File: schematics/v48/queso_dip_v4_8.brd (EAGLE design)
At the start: 41 x 50 mm, 50 parts, among them Q1 FOXSDLF/120-20, U1 PRTR5V0U2X,215, U2 PRTR5V0U2X,215, U3 PRTR5V0U2X,215, U4 PRTR5V0U2X,215, U5 PRTR5V0U2X,215, X1 USB-A-S, X2 USB-A-S, X3 USB-A-S, X4 USB-A-S

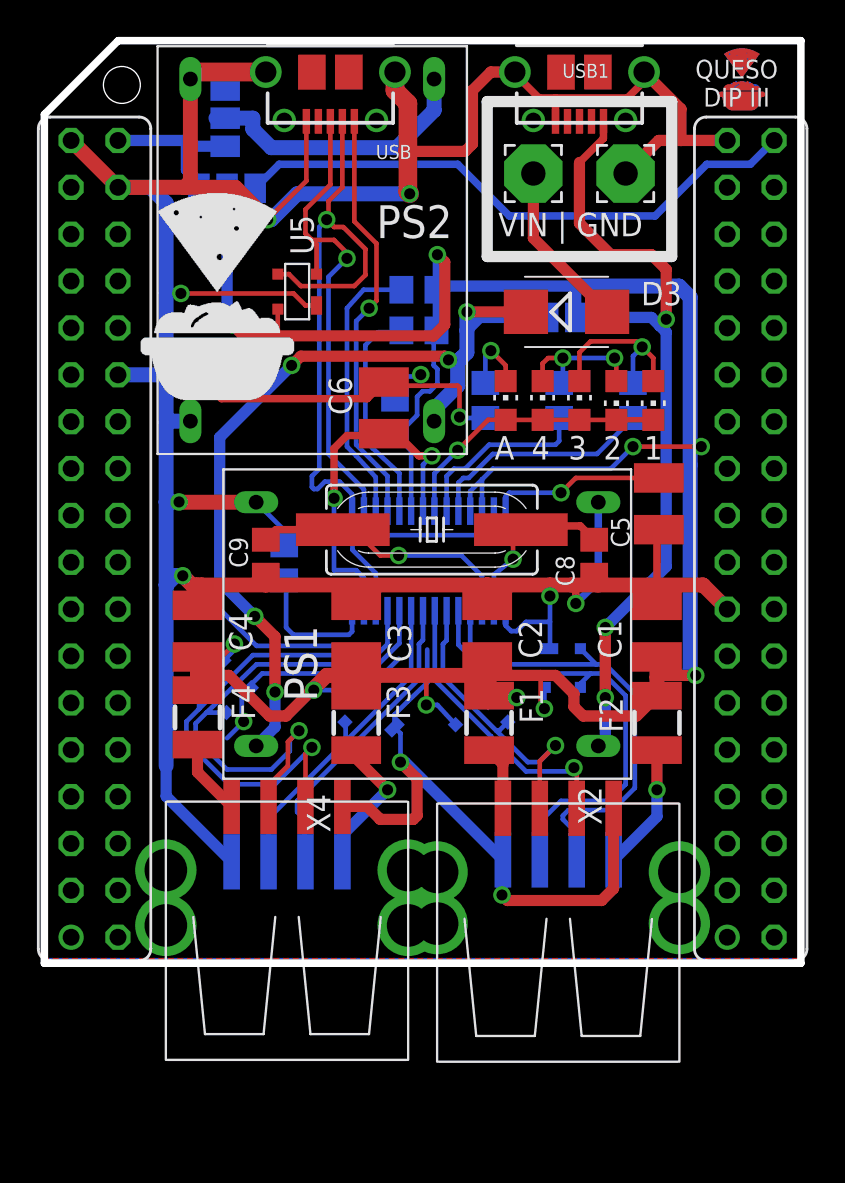
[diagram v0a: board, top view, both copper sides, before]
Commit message: fixed DRC
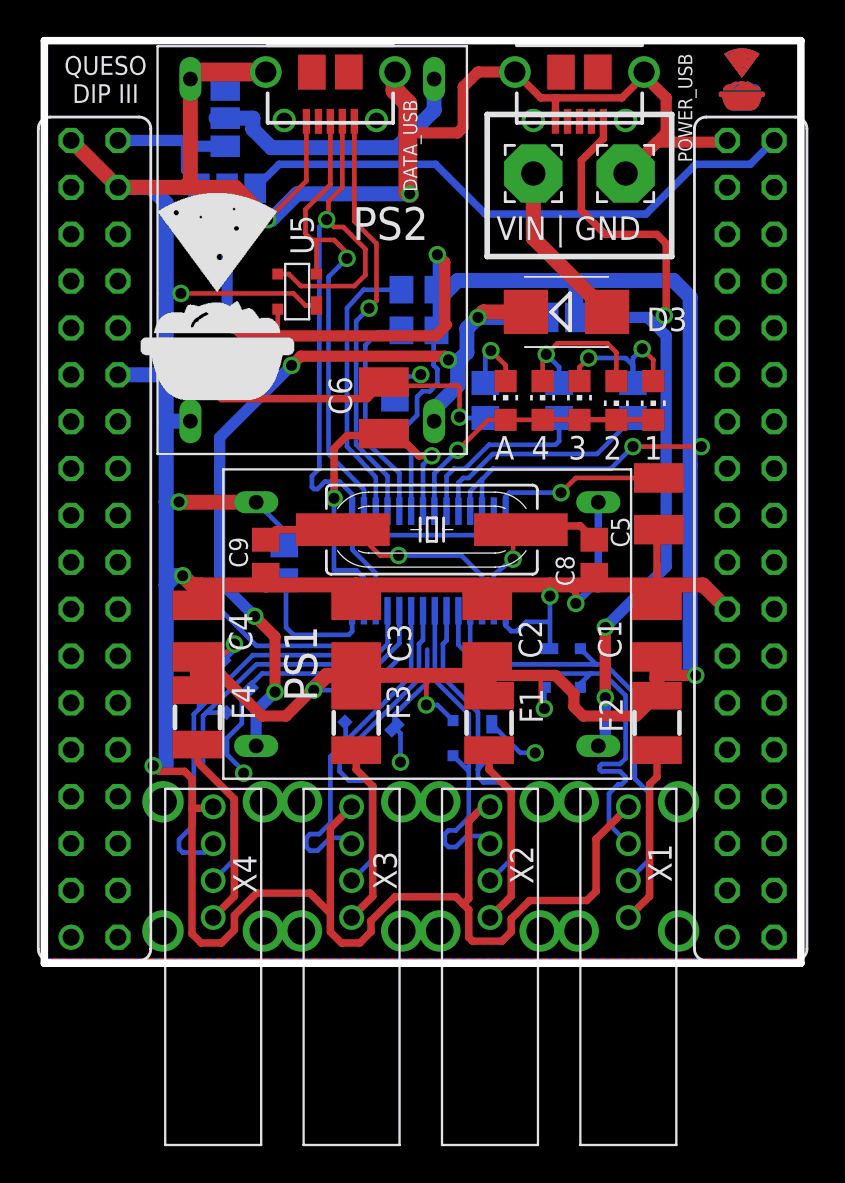
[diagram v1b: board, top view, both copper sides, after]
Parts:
- removed JP1: (no value), jumper:SJ_2
- added SJ3: (no value), SparkFun-Retired:SJ_2
- X1, X2, X3, X4: value USB-A-S -> USB-A-HU; device con-usb:USB-A-S -> con-usb:USB-A-HU
- moved X4 5.19 mm to (9.15, 1.75)
- moved X2 4.89 mm to (24.1, 1.75)
- moved X1 3.82 mm to (31.6, 1.75), flipped to the top
- moved X3 3.51 mm to (16.6, 1.75), flipped to the top
- moved U2 0.94 mm to (23.2, 12.2), turned to 270 degrees
- renumbered USB to DATA_USB, USB1 to POWER_USB
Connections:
- net VCC: now also SJ3.2; no longer JP1.2
- net VIN: now also SJ3.1; no longer JP1.1
- net VOUT: now also SJ3.3; no longer JP1.3
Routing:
- net GND: track 275.1 -> 304.3 mm
- net N$4: track 3.46 -> 10.0 mm
- net N$3: track 4.12 -> 10.7 mm
- net N$32: track 17.1 -> 21.1 mm
- net DP1: track 28.8 -> 24.9 mm, vias 1 -> 0
- net DM1: track 28.8 -> 25.1 mm, vias 1 -> 0
- net N$1: track 6.92 -> 9.71 mm, vias 1 -> 0
- net N$5: track 7.77 -> 9.92 mm, vias 1 -> 0
- net DM3: track 16.6 -> 18.4 mm, vias 1 -> 0
- net DP3: track 16.6 -> 18.3 mm, vias 1 -> 0
- net DP2: track 17.9 -> 19.5 mm
- net DM2: track 17.9 -> 19.4 mm
- net N$30: track 7.70 -> 9.18 mm, vias 2 -> 1
- net DM4: track 25.4 -> 24.0 mm
- net VCC: track 149.6 -> 151.1 mm
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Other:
- outline, holes or cut-outs redrawn
- board text added: "JKW v0.48"
- board text added: "not ordered"
- board text removed: "5V->"
- board text removed: "GND->"
- board text removed: "JKW v0.52"
- board text removed: "not ordered yet"
